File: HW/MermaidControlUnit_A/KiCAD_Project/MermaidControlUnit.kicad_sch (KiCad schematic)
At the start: 15 parts

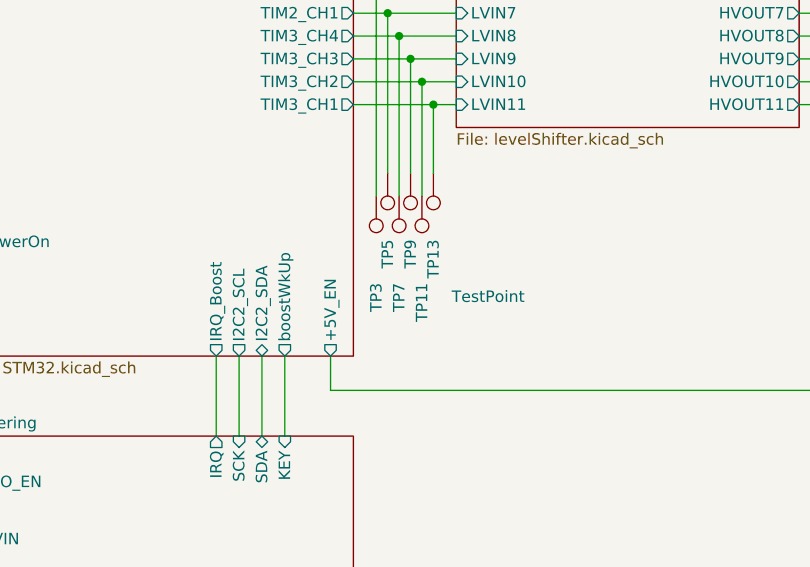
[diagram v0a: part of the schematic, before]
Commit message: schematic added, folder structure updated
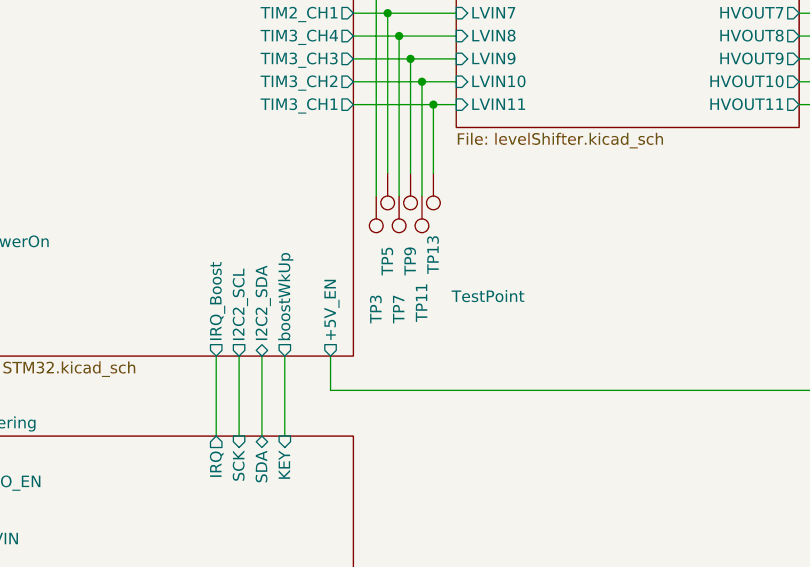
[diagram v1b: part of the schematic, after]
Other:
- company: (none) -> Aurora Dreams Mermaids
- title: (none) -> Mermaid Control Unit
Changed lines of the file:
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@@
 	(generator_version "8.0")
 	(paper "A4")
+	(title_block
+		(title "Mermaid Control Unit")
+		(date "2025-02-04")
+		(rev "A")
+		(company "Aurora Dreams Mermaids")
+		(comment 1 "Designed by: Ondrej Ruzicka")
+		(comment 4 "Hierarchy")
+	)
 	(junction
 		(at 167.64 63.5)
@@
 		(dnp no)
 		(property "Reference" "TP13"
-			(at 172.72 88.646 90)
+			(at 172.72 88.138 90)
 			(effects
 				(font
@@
 		(dnp no)
 		(property "Reference" "TP5"
-			(at 167.64 88.646 90)
+			(at 167.64 89.408 90)
 			(effects
 				(font
@@
 		(dnp no)
 		(property "Reference" "TP9"
-			(at 170.18 88.646 90)
+			(at 170.18 89.408 90)
 			(effects
 				(font
@@
 		(dnp no)
 		(property "Reference" "TP3"
-			(at 166.37 93.472 90)
+			(at 166.37 94.742 90)
 			(effects
 				(font
@@
 		(dnp no)
 		(property "Reference" "TP7"
-			(at 168.91 93.472 90)
-			(effects
-				(font
+			(at 168.91 94.742 90)
+			(effects
+				(font
